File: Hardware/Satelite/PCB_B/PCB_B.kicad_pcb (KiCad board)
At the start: 2 copper layers, 54 x 54 mm, 66 parts, among them IC1 MCP1642B-50I_MS, IC2 MCP1642B-50I_MS, J1 Conector_PCB_B-C, J2 Conector_PCB_A-B, U1 MIC5323-3.3YD5_TR, U2 ADP2108AUJ-3.3, U3 INA194, U4 MCP6001-OT, U5 INA194, U6 MCP6001-OT, U7 INA194, U8 BQ24091DGQT, U9 BQ27441DRZR-G1A

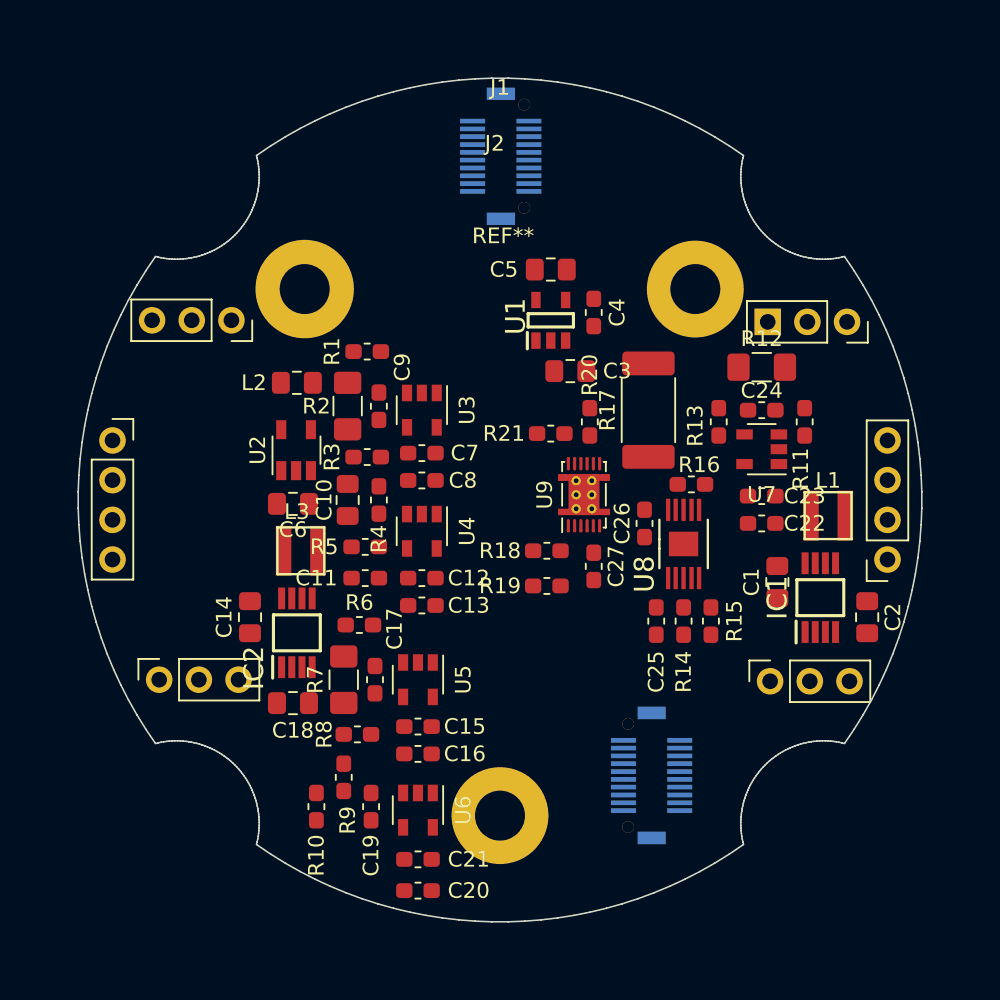
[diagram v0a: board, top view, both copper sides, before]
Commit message: PCB_B Terminado sujeto a revision
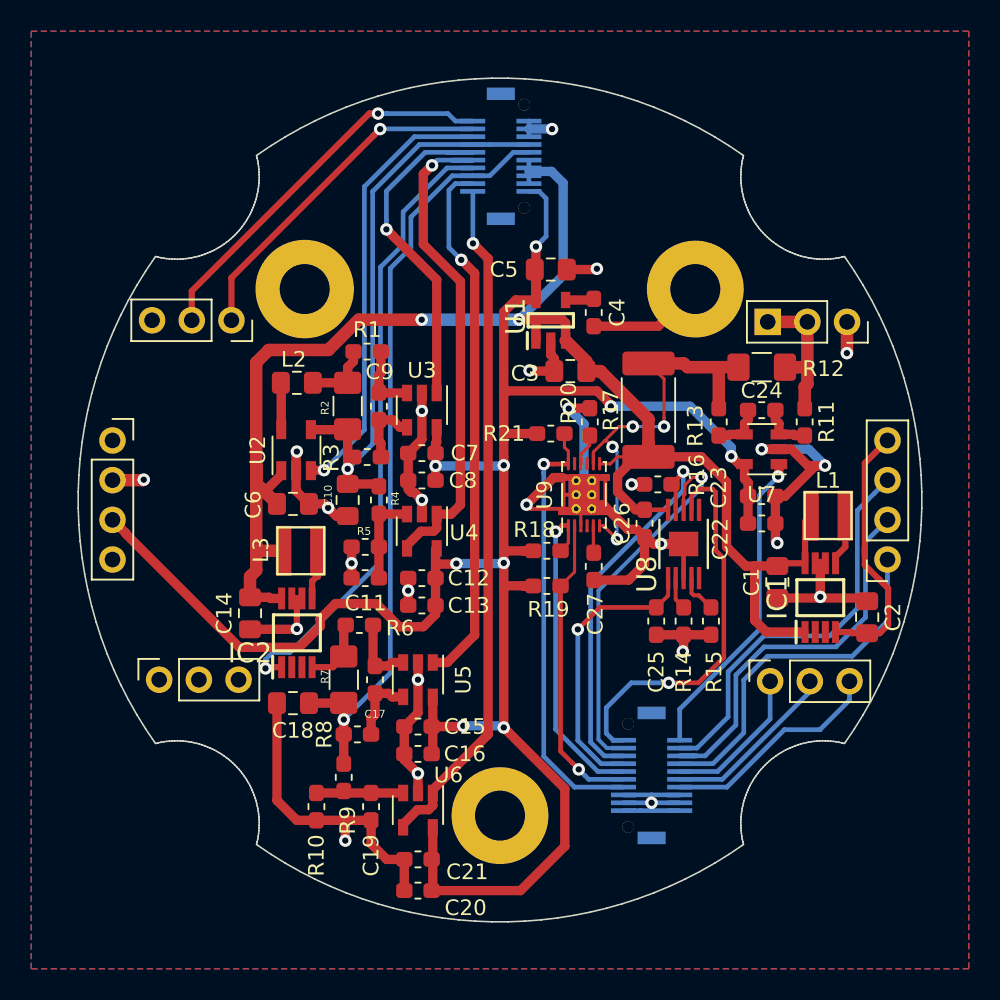
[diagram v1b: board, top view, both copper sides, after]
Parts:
- moved R16 2.15 mm to (10.1, -1.00), turned to 0 degrees
- moved C14 0.25 mm to (-16.0, 7.25)
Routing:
- net GND: track 0.00 -> 154.8 mm, vias 0 -> 25
- net +3V3_Internal: track 0.00 -> 141.0 mm, vias 0 -> 9
- net +BATT: track 0.00 -> 107.9 mm, vias 0 -> 2
- net +5V: track 0.00 -> 49.3 mm, vias 0 -> 1
- net /V_SENSE_5V: track 0.00 -> 43.8 mm, vias 0 -> 1
- net /ENABLE_5V: track 0.00 -> 40.2 mm, vias 0 -> 1
- net +3V3: track 0.00 -> 38.0 mm, vias 0 -> 1
- net /I_SENSE_5V: track 0.00 -> 34.3 mm, vias 0 -> 1
- net /V_SENSE_3V3: track 0.00 -> 32.2 mm, vias 0 -> 1
- net /ENABLE_3V3: track 0.00 -> 28.3 mm, vias 0 -> 1
- net /GPOUT: track 0.00 -> 28.2 mm, vias 0 -> 1
- net /Fuel Gauge/VBAT: track 0.00 -> 27.2 mm, vias 0 -> 4
- net /S_GLOBO: track 0.00 -> 25.8 mm
- net /S_PARACAIDAS: track 0.00 -> 25.4 mm
- net /ISET: track 0.00 -> 25.3 mm, vias 0 -> 1
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- added copper zone on B.Cu, net GND
- added copper zone on F.Cu, net GND
